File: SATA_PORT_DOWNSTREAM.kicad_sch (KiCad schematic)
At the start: 13 parts, among them CN1 HDGCYLSY-SATA-113, Q101 2N7002, Q113 2N7002, Q89 2N7002

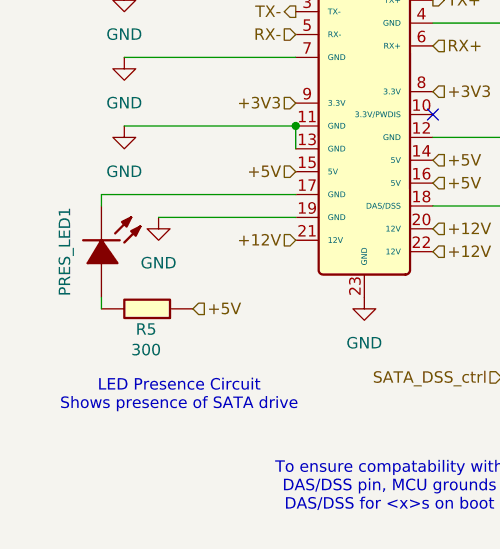
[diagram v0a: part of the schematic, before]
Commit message: Basic Function Review/Documentation of RP2354B
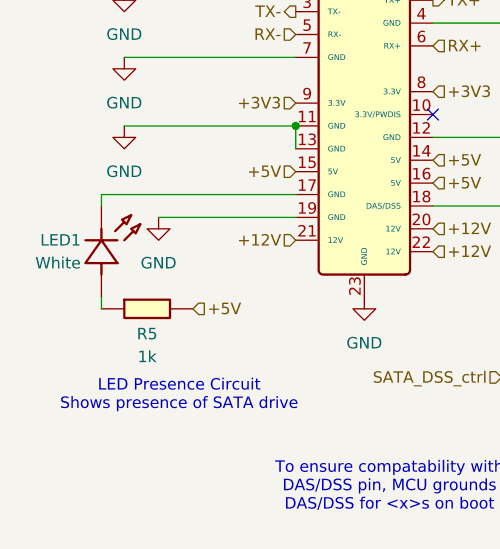
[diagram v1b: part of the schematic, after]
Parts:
- removed PRES_LED1: whiteLEDSMD, JLCImport:whiteLEDSMD, symbol JLCImport:whiteLEDSMD
- removed R5: 300, Resistor_SMD:R_0603_1608Metric, symbol JLCImport:0603WAF3000T5E
- added LED1: White, JLCImport:GL0603UW01, symbol JLCImport:GL0603UW01
- added R5: 1k, Resistor_SMD:R_0402_1005Metric, symbol JLCImport:0402WGF1001TCE
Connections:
- net +5V: now also R5.2
- net at CN1.17 (GND): now also LED1.2 (C)
- new net: LED1.1 (A), R5.1
